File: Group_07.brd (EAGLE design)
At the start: 76.2 x 77.5 mm, 29 parts, among them J1 POWER_JACKPTH_LOCK, U1 +12v, U3 TCA9546ASO16, U4 TMUX1208

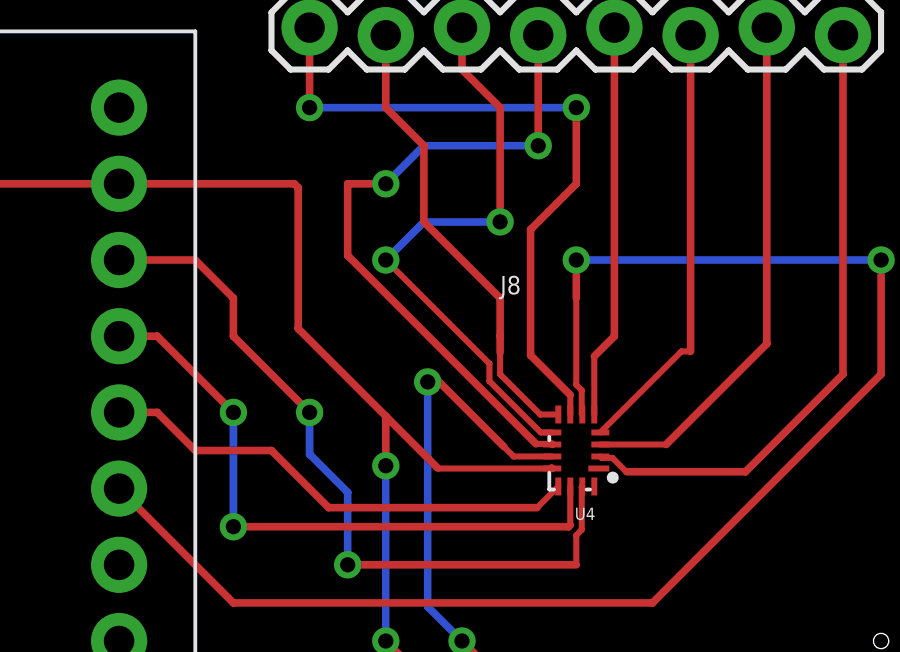
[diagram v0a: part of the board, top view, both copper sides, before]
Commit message: all fixed w/ width8
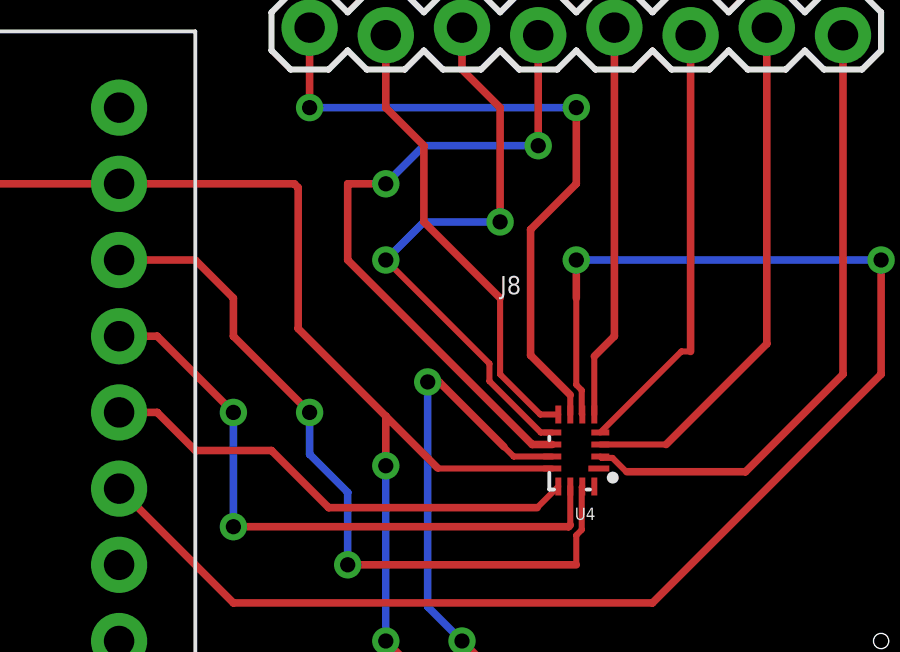
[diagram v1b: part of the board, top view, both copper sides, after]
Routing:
- net N$16: track 15.9 -> 15.4 mm
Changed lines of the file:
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@@
 <wire x1="66.04" y1="49.53" x2="66.04" y2="45.72" width="0.254" layer="1"/>
 <wire x1="66.04" y1="45.72" x2="66.04" y2="44.03" width="0.254" layer="1"/>
-<wire x1="57.658" y1="61.976" x2="59.817" y2="59.817" width="0.254" layer="1"/>
+<wire x1="59.817" y1="59.817" x2="57.658" y2="61.976" width="0.254" layer="1"/>
 <wire x1="6.858" y1="44.45" x2="6.858" y2="41.656" width="0.254" layer="1"/>
 <via x="6.858" y="41.656" extent="1-16" drill="0.508"/>
@@
 <wire x1="7.62" y1="31.75" x2="7.62" y2="15.24" width="0.254" layer="16"/>
 <wire x1="8.509" y1="11.811" x2="10.789" y2="11.811" width="0.254" layer="1"/>
-<wire x1="59.817" y1="59.817" x2="60.1424" y2="59.4916" width="0.2032" layer="1"/>
-<wire x1="60.1424" y1="59.4916" x2="61.43" y2="59.4916" width="0.2032" layer="1"/>
-<wire x1="61.43" y1="59.4916" x2="61.43" y2="59.49" width="0" layer="19" extent="1-1"/>
+<wire x1="61.43" y1="59.49" x2="60.144" y2="59.49" width="0.2032" layer="1"/>
+<wire x1="60.144" y1="59.49" x2="59.817" y2="59.817" width="0.2032" layer="1"/>
 </signal>
 <signal name="N$1">
@@
 <vertex x="76.2" y="0"/>
 </polygon>
-<wire x1="61.43" y1="59.09" x2="61.4094" y2="59.1106" width="0.254" layer="1"/>
 <wire x1="55.88" y1="60.833" x2="57.6024" y2="59.1106" width="0.254" layer="1"/>
 <wire x1="55.88" y1="60.833" x2="52.959" y2="63.754" width="0.254" layer="1"/>
@@
 <contactref element="J8" pad="4"/>
 <contactref element="U4" pad="10"/>
-<wire x1="61.4094" y1="59.9106" x2="61.43" y2="59.89" width="0.254" layer="1"/>
-<wire x1="54.61" y1="66.18786875" x2="60.88726875" y2="59.9106" width="0.254" layer="1"/>
-<wire x1="54.61" y1="66.18786875" x2="54.61" y2="68.58" width="0.254" layer="1"/>
-<wire x1="54.61" y1="68.58" x2="55.88" y2="68.58" width="0.254" layer="1"/>
+<wire x1="55.88" y1="68.58" x2="54.61" y2="68.58" width="0.254" layer="1"/>
 <via x="55.88" y="68.58" extent="1-16" drill="0.508"/>
 <wire x1="55.88" y1="68.58" x2="57.15" y2="69.85" width="0.254" layer="16"/>
@@
 <wire x1="60.96" y1="69.85" x2="60.96" y2="73.533" width="0.254" layer="1"/>
 <wire x1="57.15" y1="69.85" x2="60.96" y2="69.85" width="0.254" layer="16"/>
-<wire x1="60.88726875" y1="59.9106" x2="61.4094" y2="59.9106" width="0.2032" layer="1"/>
+<wire x1="60.76" y1="59.89" x2="61.43" y2="59.89" width="0.254" layer="1"/>
+<wire x1="54.61" y1="68.58" x2="54.61" y2="66.04" width="0.254" layer="1"/>
+<wire x1="54.61" y1="66.04" x2="60.76" y2="59.89" width="0.254" layer="1"/>
 </signal>
 <signal name="N$15">
@@
 <wire x1="59.69" y1="67.31" x2="59.69" y2="71.12" width="0.254" layer="1"/>
 <wire x1="55.88" y1="66.04" x2="59.3344" y2="62.5856" width="0.2032" layer="1"/>
-<wire x1="59.3344" y1="62.5856" x2="59.3344" y2="62.0022875" width="0.2032" layer="1"/>
-<wire x1="61.0450875" y1="60.2916" x2="61.43" y2="60.2916" width="0.2032" layer="1"/>
-<wire x1="59.3344" y1="62.0022875" x2="61.0450875" y2="60.2916" width="0.2032" layer="1"/>
-<wire x1="61.43" y1="60.2916" x2="61.43" y2="60.29" width="0" layer="19" extent="1-1"/>
+<wire x1="59.3344" y1="62.0022875" x2="59.3344" y2="62.5856" width="0.2032" layer="1"/>
+<wire x1="61.43" y1="60.29" x2="61.0466875" y2="60.29" width="0.2032" layer="1"/>
+<wire x1="61.0466875" y1="60.29" x2="59.3344" y2="62.0022875" width="0.2032" layer="1"/>
 </signal>
 <signal name="N$16">
 <contactref element="J8" pad="2"/>
 <contactref element="U4" pad="8"/>
-<wire x1="59.69" y1="64.77" x2="59.69" y2="63.5" width="0.254" layer="1"/>
-<wire x1="59.69" y1="62.957" x2="59.69" y2="63.5" width="0.254" layer="1"/>
 <wire x1="57.15" y1="69.85" x2="55.88" y2="71.12" width="0.254" layer="1"/>
 <wire x1="55.88" y1="71.12" x2="55.88" y2="73.533" width="0.254" layer="1"/>
-<wire x1="59.69" y1="64.77" x2="57.15" y2="67.31" width="0.254" layer="1"/>
+<wire x1="57.15" y1="67.31" x2="59.69" y2="64.77" width="0.254" layer="1"/>
 <wire x1="57.15" y1="67.31" x2="57.15" y2="69.85" width="0.254" layer="1"/>
-<wire x1="59.69" y1="63.5" x2="59.69" y2="62.23" width="0.2032" layer="1"/>
 <wire x1="59.69" y1="62.23" x2="61.03" y2="60.89" width="0.2032" layer="1"/>
 <wire x1="61.03" y1="60.89" x2="61.63" y2="60.89" width="0.2032" layer="1"/>
+<wire x1="59.69" y1="64.77" x2="59.69" y2="62.23" width="0.2032" layer="1"/>
 </signal>
 <signal name="N$17">

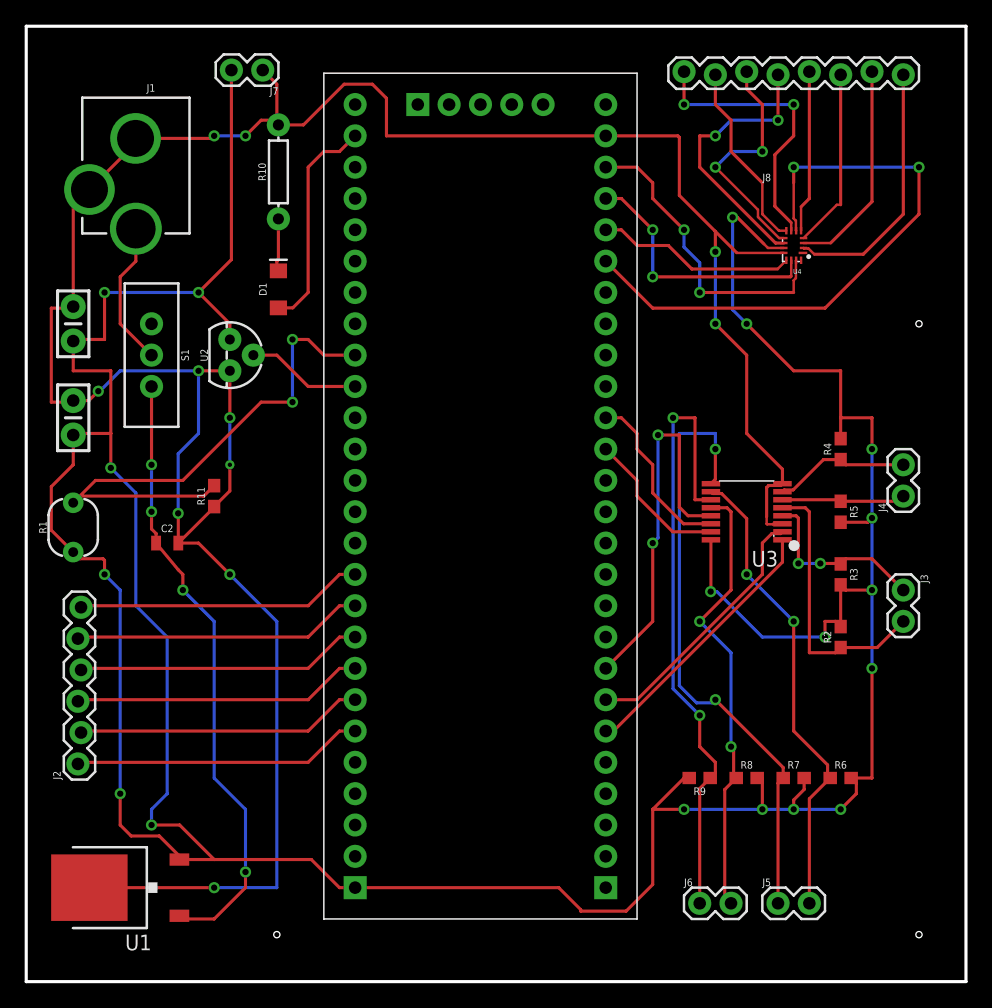
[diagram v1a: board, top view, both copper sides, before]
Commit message: Disposizione modificata
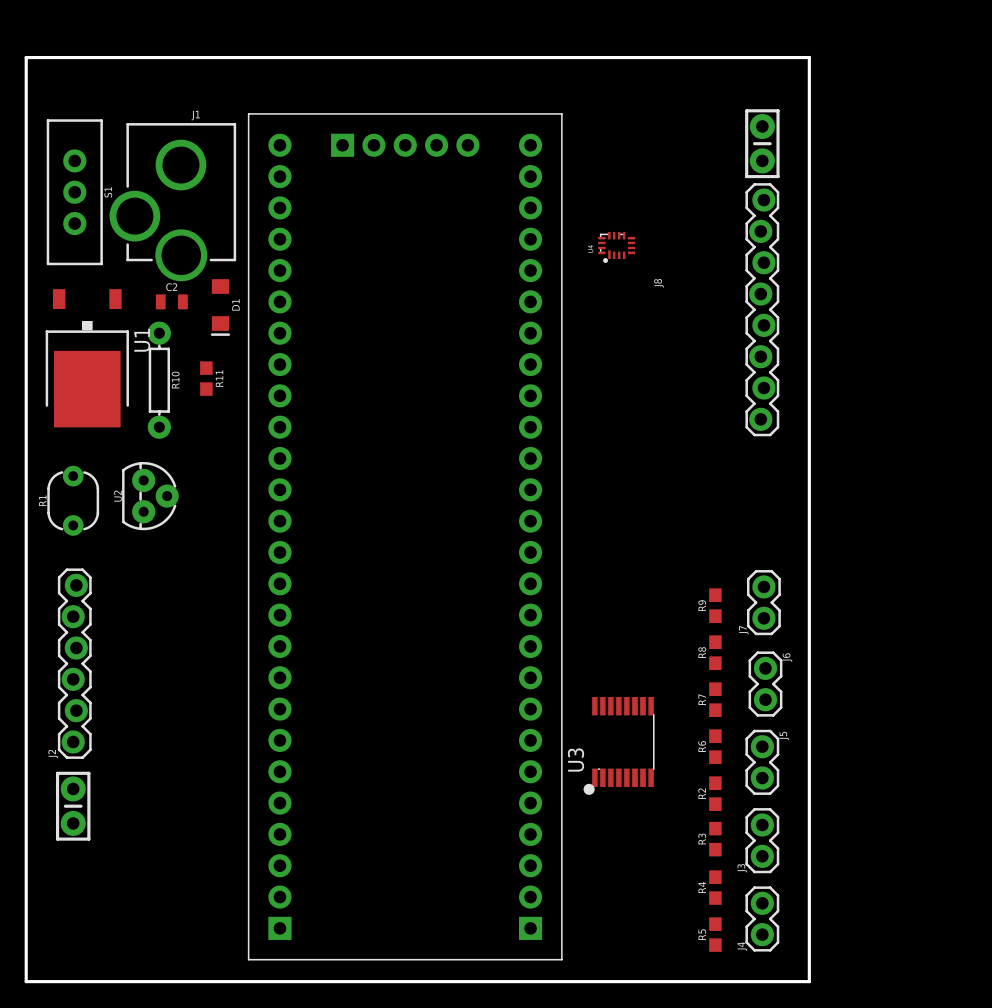
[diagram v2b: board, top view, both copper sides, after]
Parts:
- moved J7 60.2 mm to (59.8, 29.5), turned to 90 degrees
- moved C1 60.1 mm to (59.7, 67.9)
- moved U1 43.0 mm to (4.95, 50.5), turned to 180 degrees
- moved C3 39.1 mm to (3.81, 14.2)
- moved J4 37.4 mm to (59.7, 3.81)
- moved R4 37.0 mm to (55.9, 7.62)
- moved R5 35.8 mm to (55.9, 3.81), turned to 90 degrees
- moved J3 24.4 mm to (59.7, 10.2), turned to 90 degrees
- moved R3 23.7 mm to (55.9, 11.6), turned to 90 degrees
- moved U3 21.2 mm to (48.4, 19.4), turned to 90 degrees
- moved J6 19.8 mm to (59.9, 25.4), turned to 270 degrees
- moved C2 19.6 mm to (11.8, 55.1)
- moved R10 19.5 mm to (10.8, 48.8), turned to 270 degrees
- moved R2 16.3 mm to (55.9, 15.2)
- moved S1 14.6 mm to (3.94, 64.0)
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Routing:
- net 5V: track 298.5 -> 0.00 mm, vias 18 -> 0
- net GND: track 216.7 -> 0.00 mm, vias 11 -> 0
- net I2C_SDA_3: track 51.0 -> 0.00 mm, vias 2 -> 0
- net 12V: track 50.2 -> 0.00 mm, vias 4 -> 0
- net I2C_SDA_2: track 50.2 -> 0.00 mm, vias 2 -> 0
- net MUX_OUT/1.4C: track 49.3 -> 0.00 mm, vias 2 -> 0
- net PHOTO_OUT: track 43.9 -> 0.00 mm, vias 2 -> 0
- net I2C_SCL_2: track 38.6 -> 0.00 mm, vias 2 -> 0
- net I2C_SCL_3: track 36.8 -> 0.00 mm, vias 2 -> 0
- net I2C_A2: track 31.1 -> 0.00 mm, vias 2 -> 0
- net MUX_A0/1.3C: track 25.1 -> 0.00 mm, vias 2 -> 0
- net N$8: track 23.6 -> 0.00 mm
- net N$4: track 23.6 -> 0.00 mm
- net N$6: track 23.6 -> 0.00 mm
- net N$5: track 23.3 -> 0.00 mm
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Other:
- board size 76.2 x 77.5 mm -> 63.5 x 74.9 mm
